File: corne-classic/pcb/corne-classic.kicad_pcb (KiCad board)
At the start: 2 copper layers, 152.8 x 92.2 mm, 100 parts, among them J1 MJ-4PP-9, J2 OLED, J3 LED, P1 i2c-pin, P2 i2c-pin, SW1 SW_PUSH, SW10 SW_PUSH, SW11 SW_PUSH, SW12 SW_PUSH, SW13 SW_PUSH, SW14 SW_PUSH, SW15 SW_PUSH, SW16 SW_PUSH, SW17 SW_PUSH, SW18 SW_PUSH, SW19 SW_PUSH, SW2 SW_PUSH, SW20 SW_PUSH, SW21 SW_PUSH, SW22 SW_PUSH, SW3 SW_PUSH, SW4 SW_PUSH, SW5 SW_PUSH, SW6 SW_PUSH, SW7 SW_PUSH, SW8 SW_PUSH, SW9 SW_PUSH, U1 ProMicro

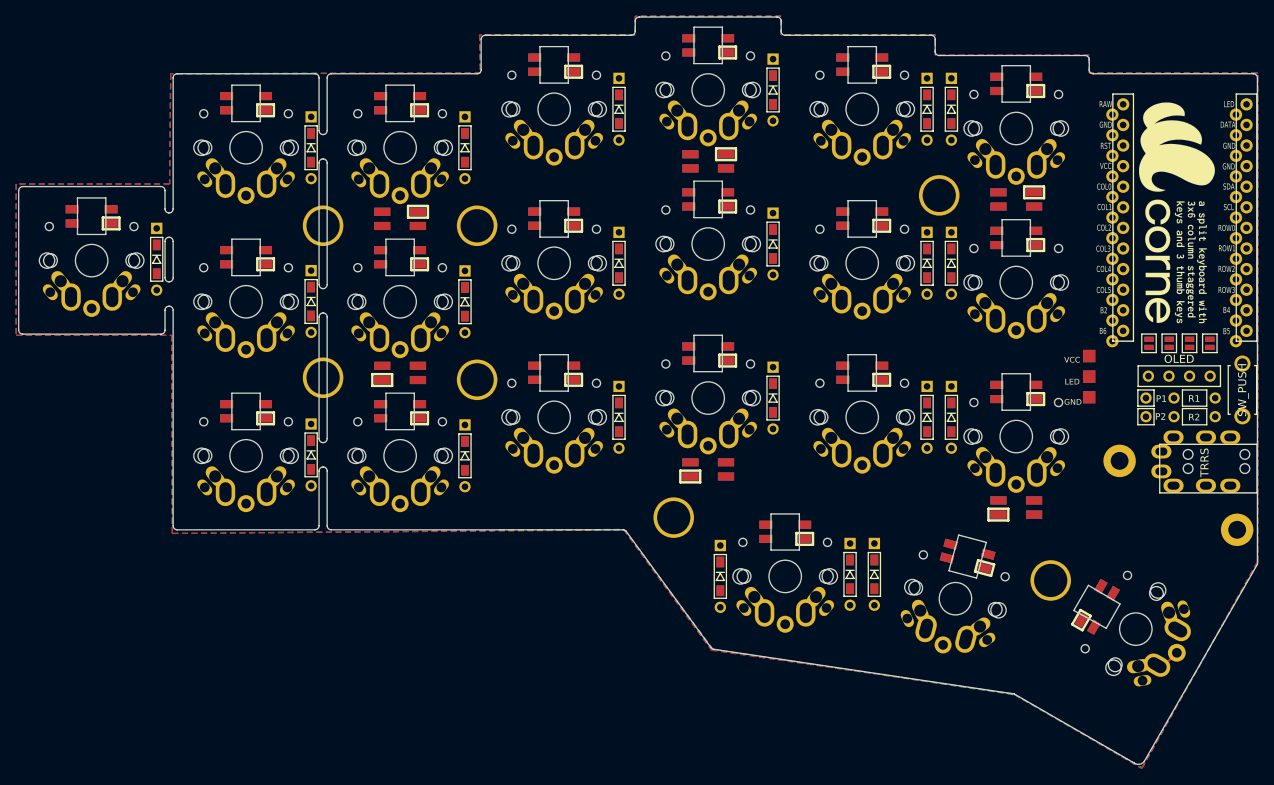
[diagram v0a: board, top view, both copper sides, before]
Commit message: updated files
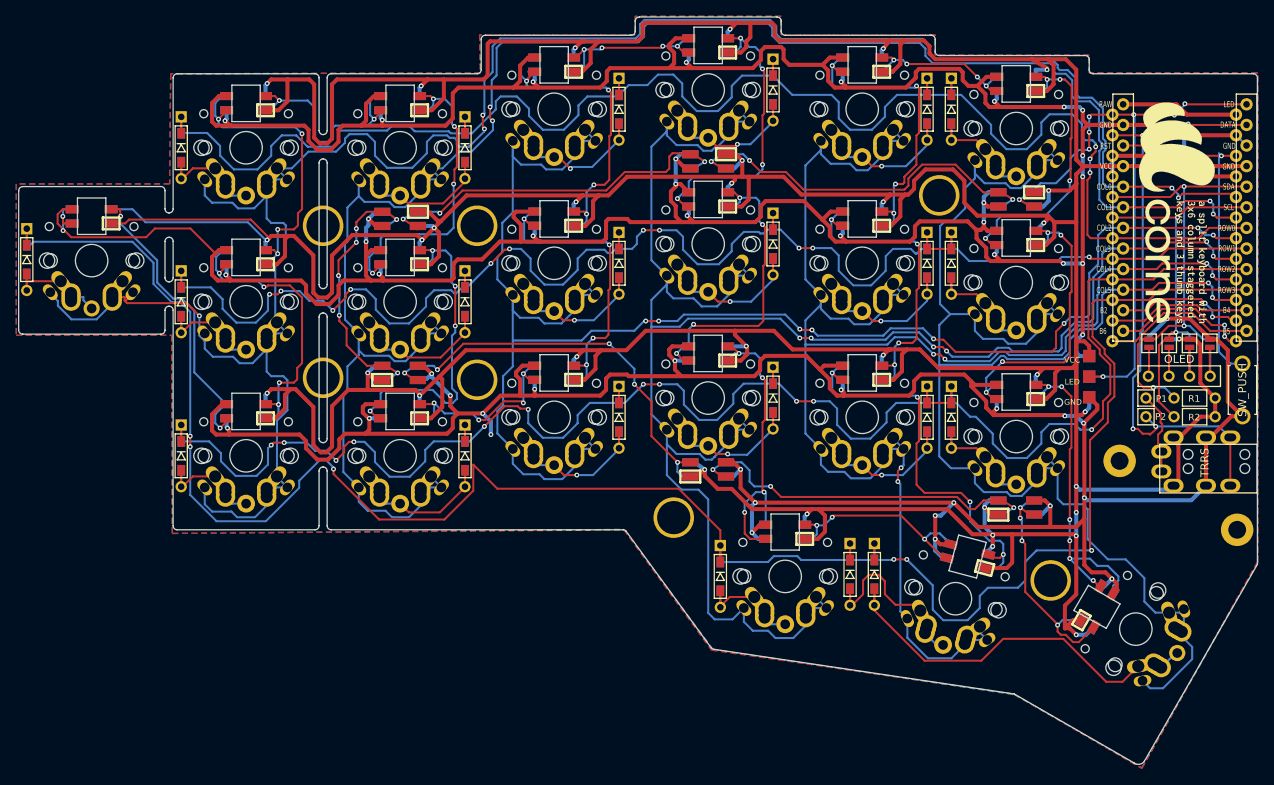
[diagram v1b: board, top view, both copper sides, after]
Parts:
- SW21: footprint kbd:MX_ALPS_PG1350_noLed -> kbd:MX_ALPS_PG1350_noLed_1.75u
- moved D22 16.0 mm to (42.9, 90.9)
- moved D13 16.0 mm to (62.0, 115.1)
- moved D7 16.0 mm to (62.0, 96.1)
- moved D1 16.0 mm to (62.0, 77.1)
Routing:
- net GND: track 0.00 -> 826.8 mm, vias 0 -> 50
- net VCC: track 0.00 -> 802.4 mm, vias 0 -> 33
- net col0: track 0.00 -> 280.4 mm, vias 0 -> 5
- net row3: track 0.00 -> 257.9 mm, vias 0 -> 6
- net col3: track 0.00 -> 229.7 mm, vias 0 -> 6
- net col1: track 0.00 -> 224.5 mm, vias 0 -> 4
- net row2: track 0.00 -> 215.8 mm, vias 0 -> 11
- net row0: track 0.00 -> 205.5 mm, vias 0 -> 3
- net col2: track 0.00 -> 200.7 mm, vias 0 -> 8
- net col4: track 0.00 -> 198.4 mm, vias 0 -> 6
- net row1: track 0.00 -> 191.7 mm, vias 0 -> 11
- net col5: track 0.00 -> 191.4 mm, vias 0 -> 2
- net LED: track 0.00 -> 77.7 mm, vias 0 -> 8
- net data: track 0.00 -> 75.1 mm, vias 0 -> 5
- net SDA: track 0.00 -> 54.9 mm, vias 0 -> 3
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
